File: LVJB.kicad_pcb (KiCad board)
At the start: 2 copper layers, 125 x 45 mm, 18 parts, among them J1 Section H1, J10 Section F, J11 Section E1, J12 Section E2, J13 Section E3, J14 Section T1A, J2 Section A1, J3 Section A2, J4 Section A3, J5 Section A4, J6 Section M, J7 Section B1, J8 Section B2, J9 Section K

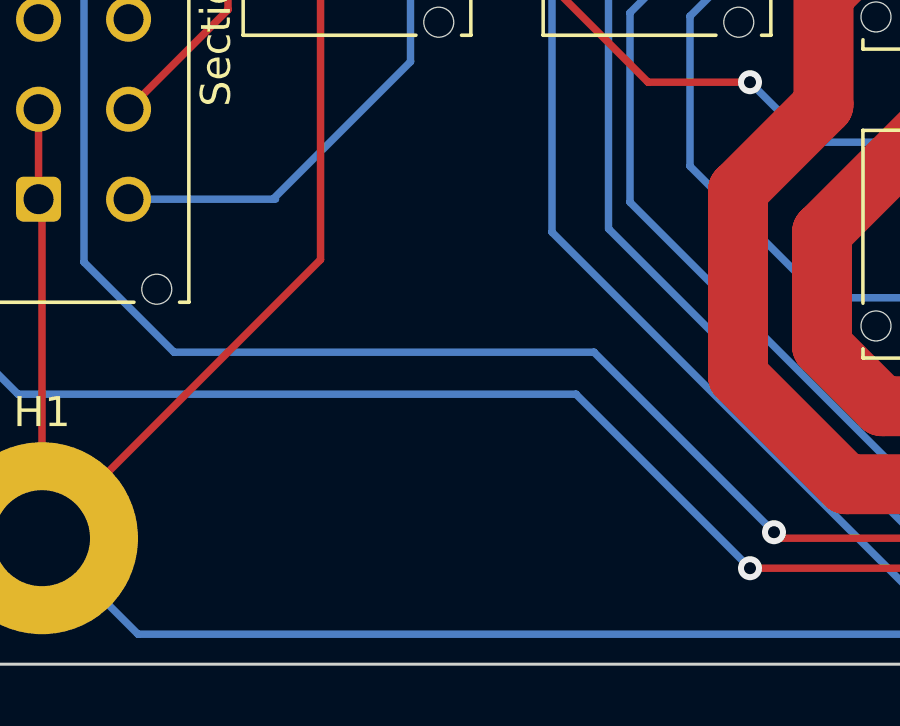
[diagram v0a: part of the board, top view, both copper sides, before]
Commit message: added art
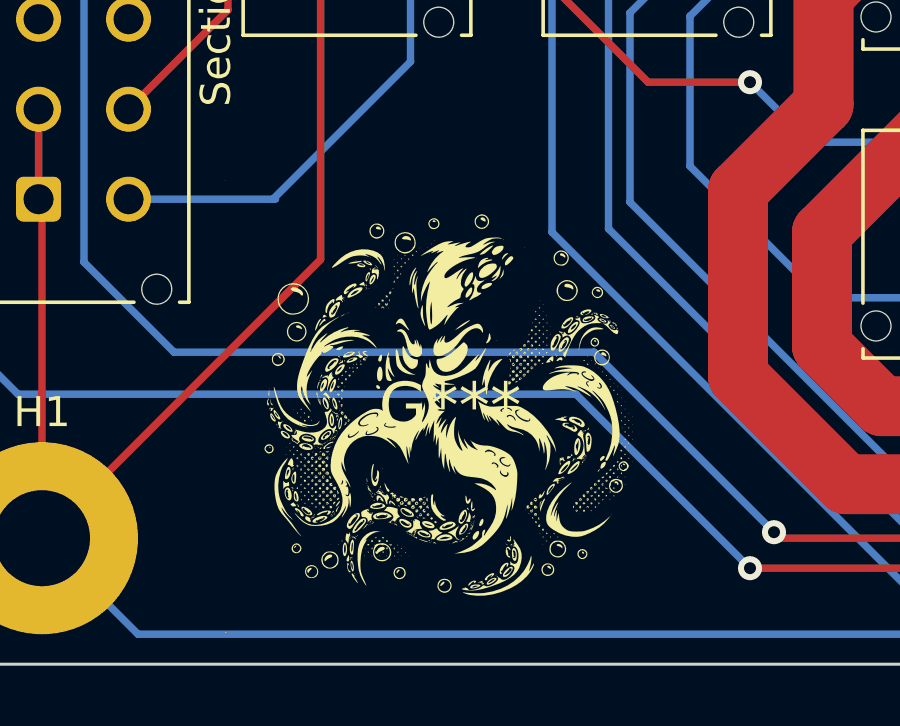
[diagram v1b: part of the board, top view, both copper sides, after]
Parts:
- added G***: LOGO, LOGO, F.Cu at (106.8, 87.4)
